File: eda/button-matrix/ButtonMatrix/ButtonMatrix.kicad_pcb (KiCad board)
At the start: 2 copper layers, 87.2 x 87.2 mm, 54 parts, among them J1 Conn_01x12, J2 Conn_01x12, SW1 SW_Omron_B3FS, SW10 SW_Omron_B3FS, SW11 SW_Omron_B3FS, SW12 SW_Omron_B3FS, SW13 SW_Omron_B3FS, SW14 SW_Omron_B3FS, SW15 SW_Omron_B3FS, SW16 SW_Omron_B3FS, SW2 SW_Omron_B3FS, SW3 SW_Omron_B3FS, SW4 SW_Omron_B3FS, SW5 SW_Omron_B3FS, SW6 SW_Omron_B3FS, SW7 SW_Omron_B3FS, SW8 SW_Omron_B3FS, SW9 SW_Omron_B3FS

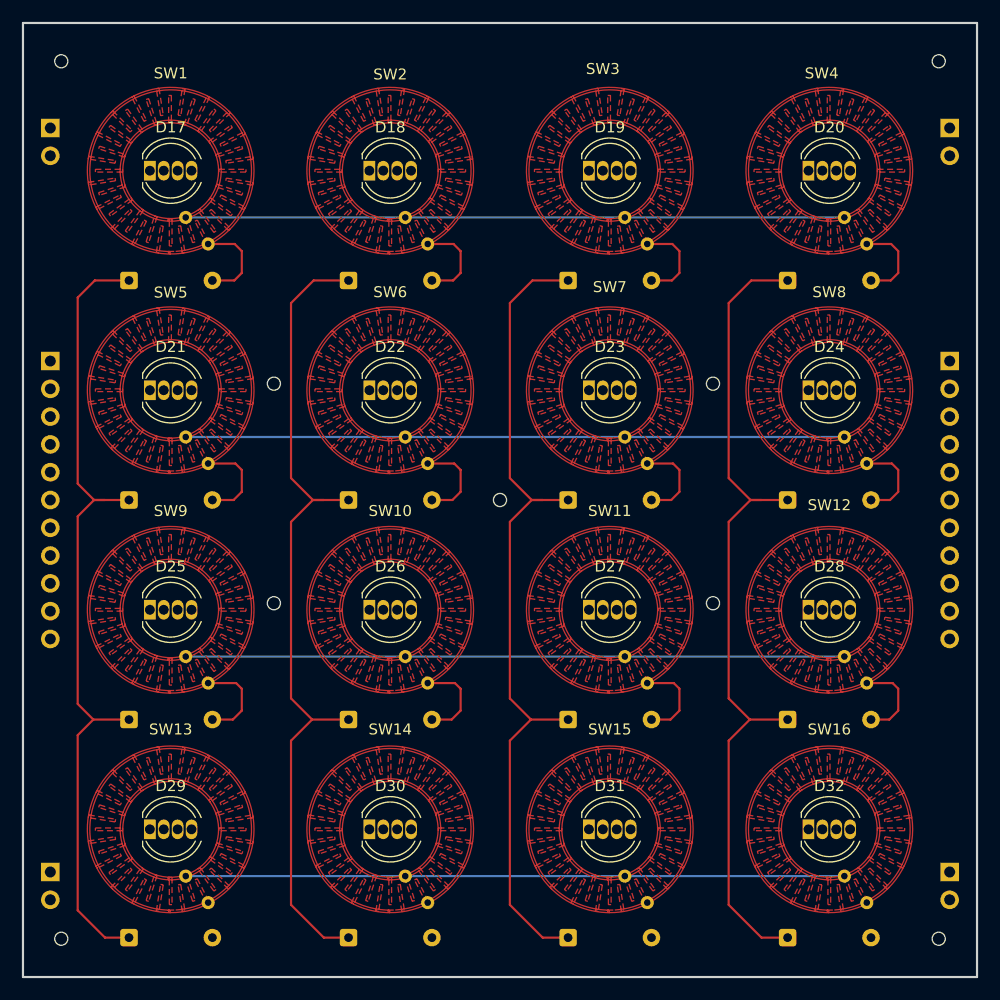
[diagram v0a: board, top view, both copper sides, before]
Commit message: - Updated PCB more
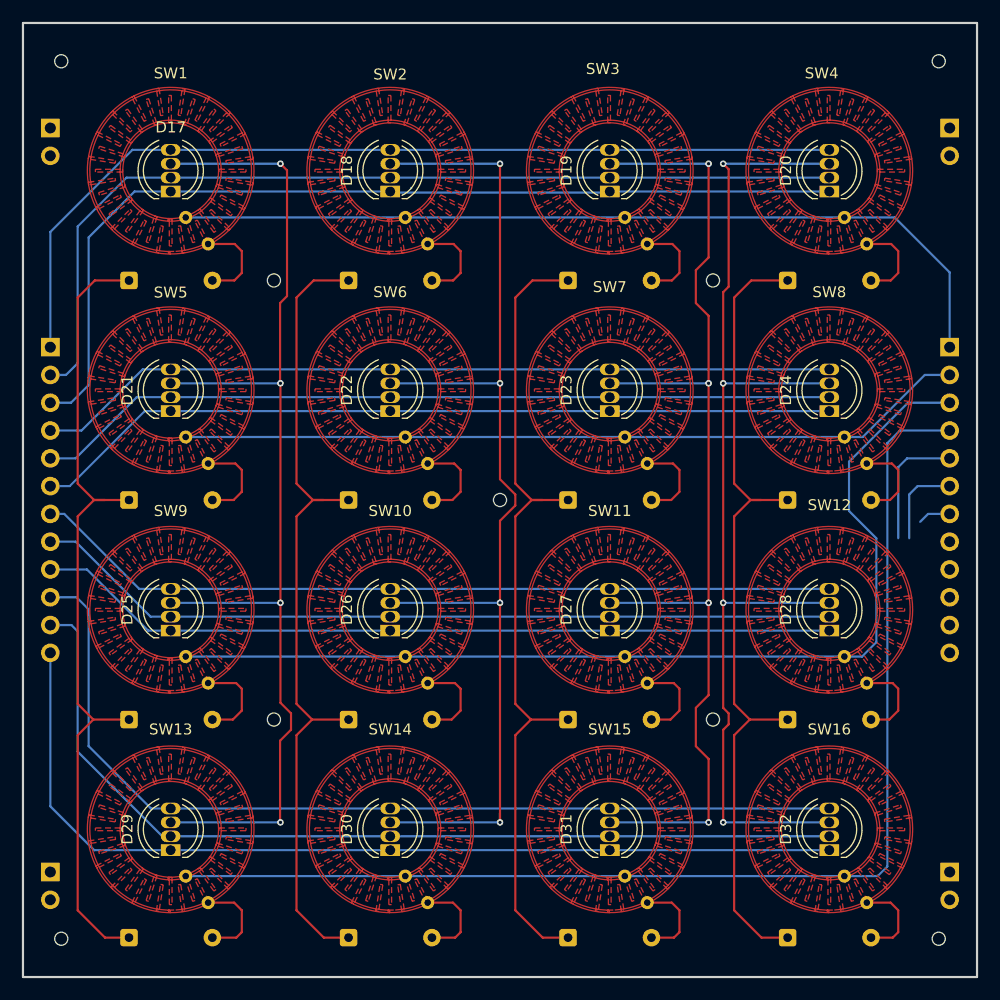
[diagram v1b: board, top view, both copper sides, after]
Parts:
- J1, J2: footprint Connector_PinHeader_2.54mm:PinHeader_1x11_P2.54mm_Vertical -> Connector_PinHeader_2.54mm:PinHeader_1x12_P2.54mm_Vertical
- moved D17 2.69 mm to (141.5, 74.8), turned to 90 degrees
- moved D18 2.69 mm to (161.6, 74.8), turned to 90 degrees
- moved D19 2.69 mm to (181.6, 74.8), turned to 90 degrees
- moved D20 2.69 mm to (201.7, 74.8), turned to 90 degrees
- moved D21 2.69 mm to (141.5, 94.9), turned to 90 degrees
- moved D22 2.69 mm to (161.6, 94.9), turned to 90 degrees
- moved D23 2.69 mm to (181.6, 94.9), turned to 90 degrees
- moved D24 2.69 mm to (201.7, 94.9), turned to 90 degrees
- moved D25 2.69 mm to (141.5, 114.9), turned to 90 degrees
- moved D26 2.69 mm to (161.6, 114.9), turned to 90 degrees
- moved D27 2.69 mm to (181.6, 114.9), turned to 90 degrees
- moved D28 2.69 mm to (201.7, 114.9), turned to 90 degrees
- moved D29 2.69 mm to (141.5, 135.0), turned to 90 degrees
- moved D30 2.69 mm to (161.6, 135.0), turned to 90 degrees
- moved D31 2.69 mm to (181.6, 135.0), turned to 90 degrees
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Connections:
- D17 pad 1: unconnected-(D17-BK-Pad1) -> /LED_B1
- D17 pad 2: unconnected-(D17-GK-Pad2) -> /LED_G1
- D17 pad 3: unconnected-(D17-A-Pad3) -> /LED_COL1
- D17 pad 4: unconnected-(D17-RK-Pad4) -> /LED_R1
- D18 pad 1: unconnected-(D18-BK-Pad1) -> /LED_B1
- D18 pad 2: unconnected-(D18-GK-Pad2) -> /LED_G1
- D18 pad 3: unconnected-(D18-A-Pad3) -> /LED_COL2
- D18 pad 4: unconnected-(D18-RK-Pad4) -> /LED_R1
- D19 pad 1: unconnected-(D19-BK-Pad1) -> /LED_B1
- D19 pad 2: unconnected-(D19-GK-Pad2) -> /LED_G1
- D19 pad 3: unconnected-(D19-A-Pad3) -> /LED_COL3
- D19 pad 4: unconnected-(D19-RK-Pad4) -> /LED_R1
- D20 pad 1: unconnected-(D20-BK-Pad1) -> /LED_B1
- D20 pad 2: unconnected-(D20-GK-Pad2) -> /LED_G1
- D20 pad 3: unconnected-(D20-A-Pad3) -> /LED_COL4
- D20 pad 4: unconnected-(D20-RK-Pad4) -> /LED_R1
- D21 pad 1: unconnected-(D21-BK-Pad1) -> /LED_B2
- D21 pad 2: unconnected-(D21-GK-Pad2) -> /LED_G2
- D21 pad 3: unconnected-(D21-A-Pad3) -> /LED_COL1
- D21 pad 4: unconnected-(D21-RK-Pad4) -> /LED_R2
- D22 pad 1: unconnected-(D22-BK-Pad1) -> /LED_B2
- D22 pad 2: unconnected-(D22-GK-Pad2) -> /LED_G2
- D22 pad 3: unconnected-(D22-A-Pad3) -> /LED_COL2
- D22 pad 4: unconnected-(D22-RK-Pad4) -> /LED_R2
- D23 pad 1: unconnected-(D23-BK-Pad1) -> /LED_B2
- D23 pad 2: unconnected-(D23-GK-Pad2) -> /LED_G2
- D23 pad 3: unconnected-(D23-A-Pad3) -> /LED_COL3
- D23 pad 4: unconnected-(D23-RK-Pad4) -> /LED_R2
- D24 pad 1: unconnected-(D24-BK-Pad1) -> /LED_B2
- D24 pad 2: unconnected-(D24-GK-Pad2) -> /LED_G2
- D24 pad 3: unconnected-(D24-A-Pad3) -> /LED_COL4
- D24 pad 4: unconnected-(D24-RK-Pad4) -> /LED_R2
- D25 pad 1: unconnected-(D25-BK-Pad1) -> /LED_B3
- D25 pad 2: unconnected-(D25-GK-Pad2) -> /LED_G3
- D25 pad 3: unconnected-(D25-A-Pad3) -> /LED_COL1
- D25 pad 4: unconnected-(D25-RK-Pad4) -> /LED_R3
- D26 pad 1: unconnected-(D26-BK-Pad1) -> /LED_B3
- D26 pad 2: unconnected-(D26-GK-Pad2) -> /LED_G3
- D26 pad 3: unconnected-(D26-A-Pad3) -> /LED_COL2
- D26 pad 4: unconnected-(D26-RK-Pad4) -> /LED_R3
- D27 pad 1: unconnected-(D27-BK-Pad1) -> /LED_B3
- D27 pad 2: unconnected-(D27-GK-Pad2) -> /LED_G3
- D27 pad 3: unconnected-(D27-A-Pad3) -> /LED_COL3
- D27 pad 4: unconnected-(D27-RK-Pad4) -> /LED_R3
- D28 pad 1: unconnected-(D28-BK-Pad1) -> /LED_B3
- D28 pad 2: unconnected-(D28-GK-Pad2) -> /LED_G3
- D28 pad 3: unconnected-(D28-A-Pad3) -> /LED_COL4
- D28 pad 4: unconnected-(D28-RK-Pad4) -> /LED_R3
- D29 pad 1: unconnected-(D29-BK-Pad1) -> /LED_B4
- D29 pad 2: unconnected-(D29-GK-Pad2) -> /LED_G4
- D29 pad 3: unconnected-(D29-A-Pad3) -> /LED_COL1
- D29 pad 4: unconnected-(D29-RK-Pad4) -> /LED_R4
- D30 pad 1: unconnected-(D30-BK-Pad1) -> /LED_B4
- D30 pad 2: unconnected-(D30-GK-Pad2) -> /LED_G4
- D30 pad 3: unconnected-(D30-A-Pad3) -> /LED_COL2
- D30 pad 4: unconnected-(D30-RK-Pad4) -> /LED_R4
- D31 pad 1: unconnected-(D31-BK-Pad1) -> /LED_B4
- D31 pad 2: unconnected-(D31-GK-Pad2) -> /LED_G4
- D31 pad 3: unconnected-(D31-A-Pad3) -> /LED_COL3
- D31 pad 4: unconnected-(D31-RK-Pad4) -> /LED_R4
- D32 pad 1: unconnected-(D32-BK-Pad1) -> /LED_B4
- D32 pad 2: unconnected-(D32-GK-Pad2) -> /LED_G4
- D32 pad 3: unconnected-(D32-A-Pad3) -> /LED_COL4
- D32 pad 4: unconnected-(D32-RK-Pad4) -> /LED_R4
- J1 pad 1: unconnected-(J1-Pin_1-Pad1) -> /SW_ROW1
- J1 pad 10: unconnected-(J1-Pin_10-Pad10) -> /LED_COL2
- J1 pad 11: unconnected-(J1-Pin_11-Pad11) -> /LED_COL3
- J1 pad 2: unconnected-(J1-Pin_2-Pad2) -> /SW_ROW2
- J1 pad 3: unconnected-(J1-Pin_3-Pad3) -> /SW_ROW3
- J1 pad 4: unconnected-(J1-Pin_4-Pad4) -> /SW_ROW4
- J1 pad 5: unconnected-(J1-Pin_5-Pad5) -> /SW_COL1
- J1 pad 6: unconnected-(J1-Pin_6-Pad6) -> /SW_COL2
- J1 pad 7: unconnected-(J1-Pin_7-Pad7) -> /SW_COL3
- J1 pad 8: unconnected-(J1-Pin_8-Pad8) -> /SW_COL4
- J1 pad 9: unconnected-(J1-Pin_9-Pad9) -> /LED_COL1
- J2 pad 1: unconnected-(J2-Pin_1-Pad1) -> /LED_R1
- J2 pad 10: unconnected-(J2-Pin_10-Pad10) -> /LED_R4
- J2 pad 11: unconnected-(J2-Pin_11-Pad11) -> /LED_G4
- J2 pad 2: unconnected-(J2-Pin_2-Pad2) -> /LED_G1
- J2 pad 3: unconnected-(J2-Pin_3-Pad3) -> /LED_B1
- J2 pad 4: unconnected-(J2-Pin_4-Pad4) -> /LED_R2
- J2 pad 5: unconnected-(J2-Pin_5-Pad5) -> /LED_G2
- J2 pad 6: unconnected-(J2-Pin_6-Pad6) -> /LED_B2
- J2 pad 7: unconnected-(J2-Pin_7-Pad7) -> /LED_R3
- J2 pad 8: unconnected-(J2-Pin_8-Pad8) -> /LED_G3
- J2 pad 9: unconnected-(J2-Pin_9-Pad9) -> /LED_B3
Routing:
- net /LED_COL2: track 0.00 -> 102.4 mm, vias 0 -> 4
- net /LED_COL1: track 0.00 -> 101.7 mm, vias 0 -> 4
- net /LED_COL4: track 0.00 -> 99.8 mm, vias 0 -> 4
- net /LED_COL3: track 0.00 -> 98.3 mm, vias 0 -> 4
- net /LED_B1: track 0.00 -> 87.2 mm
- net /LED_B4: track 0.00 -> 86.9 mm
- net /LED_R4: track 0.00 -> 86.5 mm
- net /LED_G1: track 0.00 -> 86.0 mm
- net /LED_G4: track 0.00 -> 85.6 mm
- net /LED_R1: track 0.00 -> 84.9 mm
- net /LED_B2: track 0.00 -> 74.0 mm
- net /LED_R3: track 0.00 -> 74.0 mm
- net /LED_G3: track 0.00 -> 74.0 mm
- net /LED_R2: track 0.00 -> 73.5 mm
- net /LED_G2: track 0.00 -> 73.5 mm
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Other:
- outline, holes or cut-outs redrawn
